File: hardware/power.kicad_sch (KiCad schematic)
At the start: 8 parts, among them U4 NCP565D2T33R4G, U6 SPBW06F-05

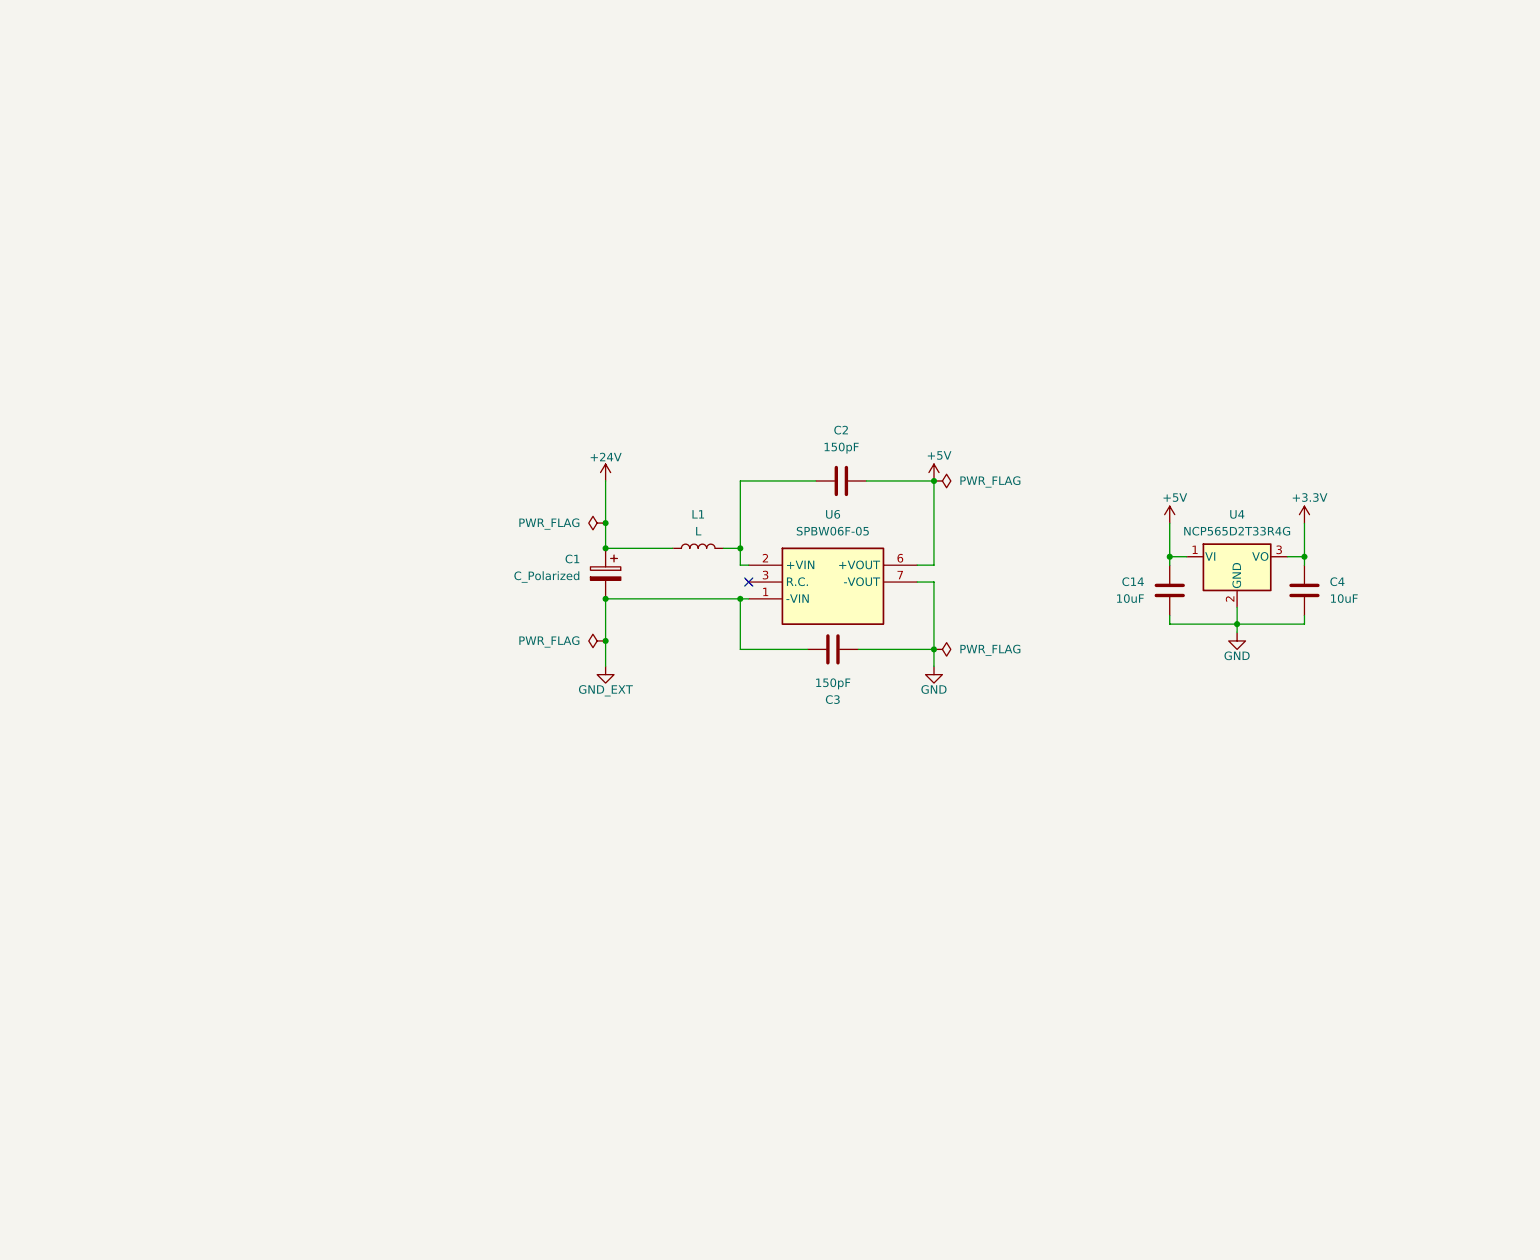
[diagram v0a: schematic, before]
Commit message: Fixes after review
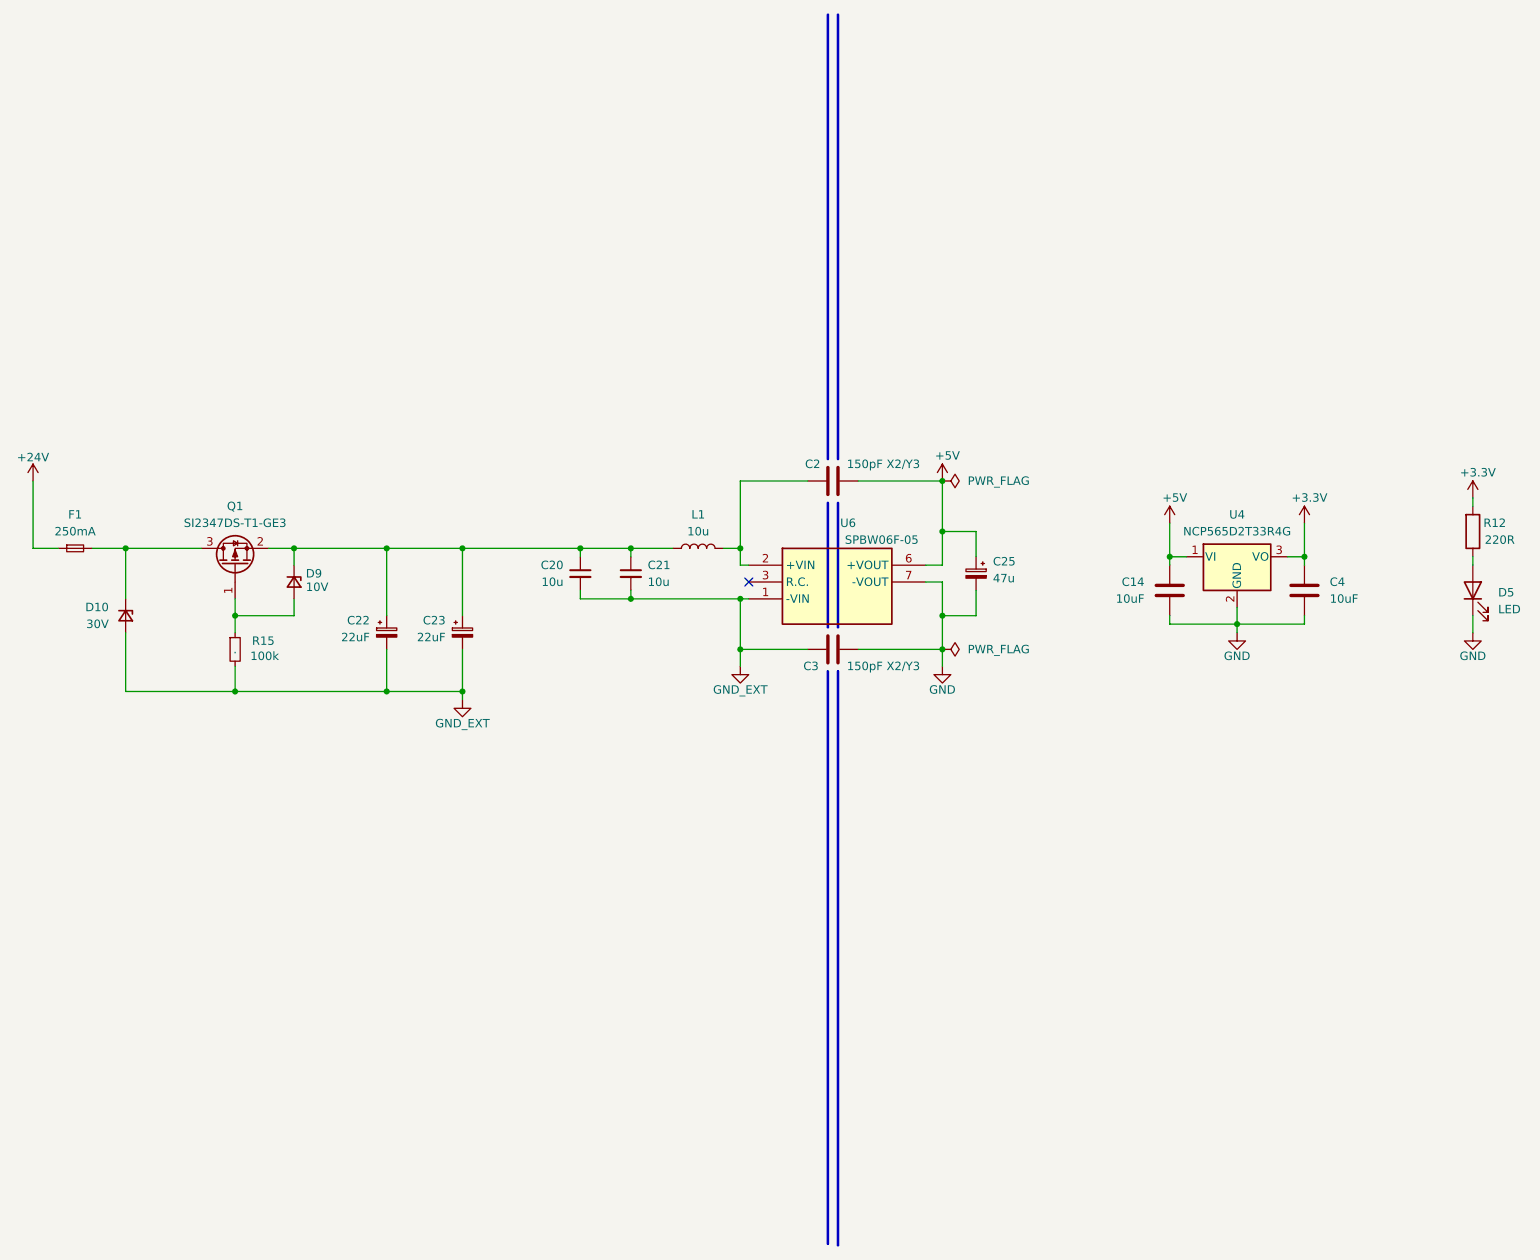
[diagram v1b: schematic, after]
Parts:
- removed C1: C_Polarized, electrolytic_cap:EEE0GA101SR, symbol Device:C_Polarized
- added C20, C21: 10u, 10uCap:CAPC3225X280N, symbol Device:C_Small
- added C22, C23: 22uF, Capacitor_SMD:CP_Elec_4x5.8, symbol Device:C_Polarized_Small
- added C25: 47u, 47uCapPolarized:EEE1AA220WR, symbol Device:C_Polarized_Small
- added D10: 30V, Diode_SMD:D_SOD-123, symbol Device:D_Zener_Small
- added D5: LED, symbol Device:LED
- added D9: 10V, Diode_SMD:D_SOD-123, symbol Device:D_Zener_Small
- added F1: 250mA, 24V250mAFuse:FUSC1608X43N, symbol Device:Fuse_Small
- added Q1: SI2347DS-T1-GE3, Package_TO_SOT_SMD:SOT-23-3, symbol Transistor_FET:Q_PMOS_GSD
- added R12: 220R, symbol Device:R
- added R15: 100k, Resistor_SMD:R_0603_1608Metric_Pad0.98x0.95mm_HandSolder, symbol Device:R_Small
- C2, C3: value 150pF -> 150pF X2/Y3; Mouser https://www.mouser.pl/ProductDetail/Vishay/VJ1206A151JXFTW1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 -> https://www.mouser.pl/ProductDetail/Knowles-Novacap/LS1808N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
- L1: value L -> 10u
- U6: Mouser Price/Stock https://www.mouser.pl/ProductDetail/MEAN-WELL/SPBW03F-05?qs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 -> https://www.mouser.pl/ProductDetail/MEAN-WELL/SPBW06F-05?qs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
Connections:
- net +24V: now also F1.1; no longer L1.1
- net +3.3V: now also R12.2
- net +5V: now also C25.1
- net GND: now also C25.2, D5.1 (K)
- net GND_EXT: now also C20.2, C21.2, C22.2, C23.2, D10.2 (A), R15.2
- new net: C20.1, C21.1, C22.1, C23.1, D9.1 (K), L1.1, Q1.2 (S)
- new net: D9.2 (A), Q1.1 (G), R15.1
- new net: D10.1 (K), F1.2, Q1.3 (D)
- new net: D5.2 (A), R12.1
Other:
- moved on the sheet: C2, U6
